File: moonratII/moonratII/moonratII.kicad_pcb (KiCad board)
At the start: 2 copper layers, 10 parts, among them Q101 IRF540N, SW101 6mm 2 Pin Tact NO, SW102 6mm 2 Pin Tact NO, SW103 6mm 2 Pin Tact NO, U101 TMP36xS

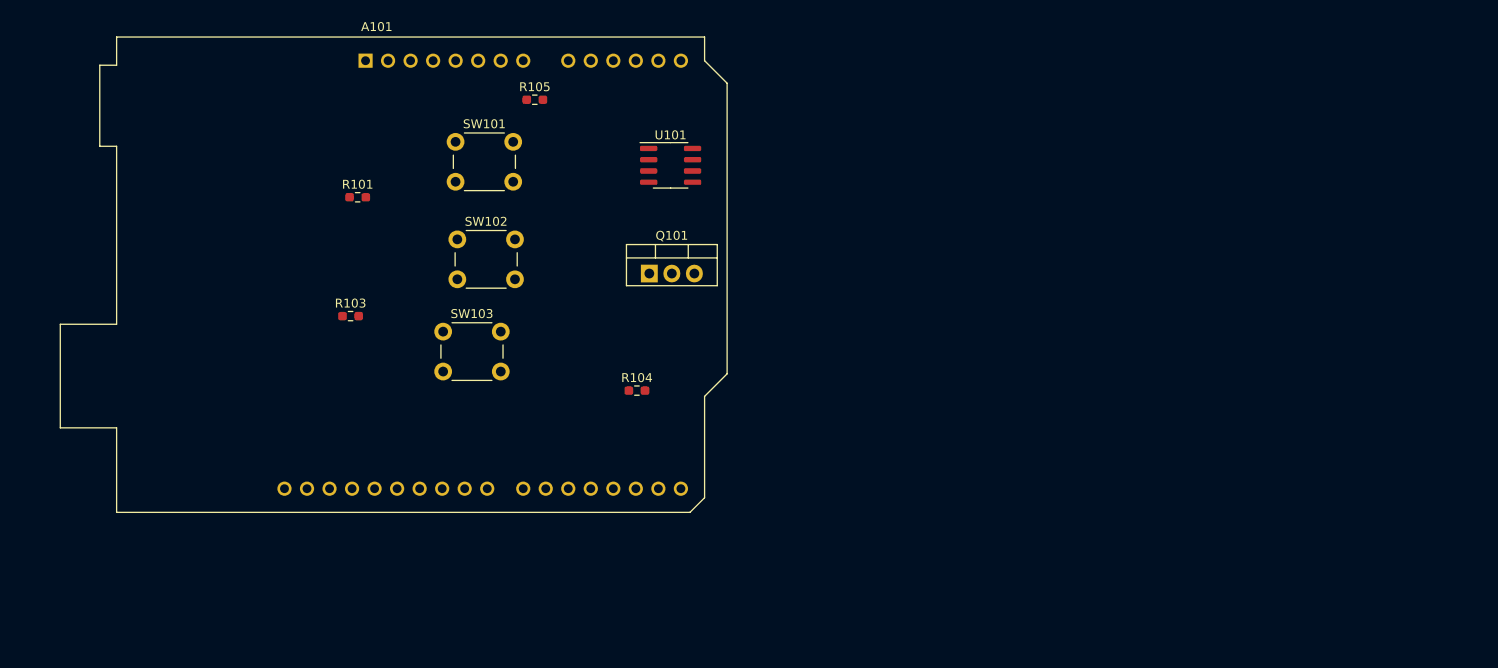
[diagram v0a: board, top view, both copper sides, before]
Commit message: Pull in parts to PCB. Make some initial placement.
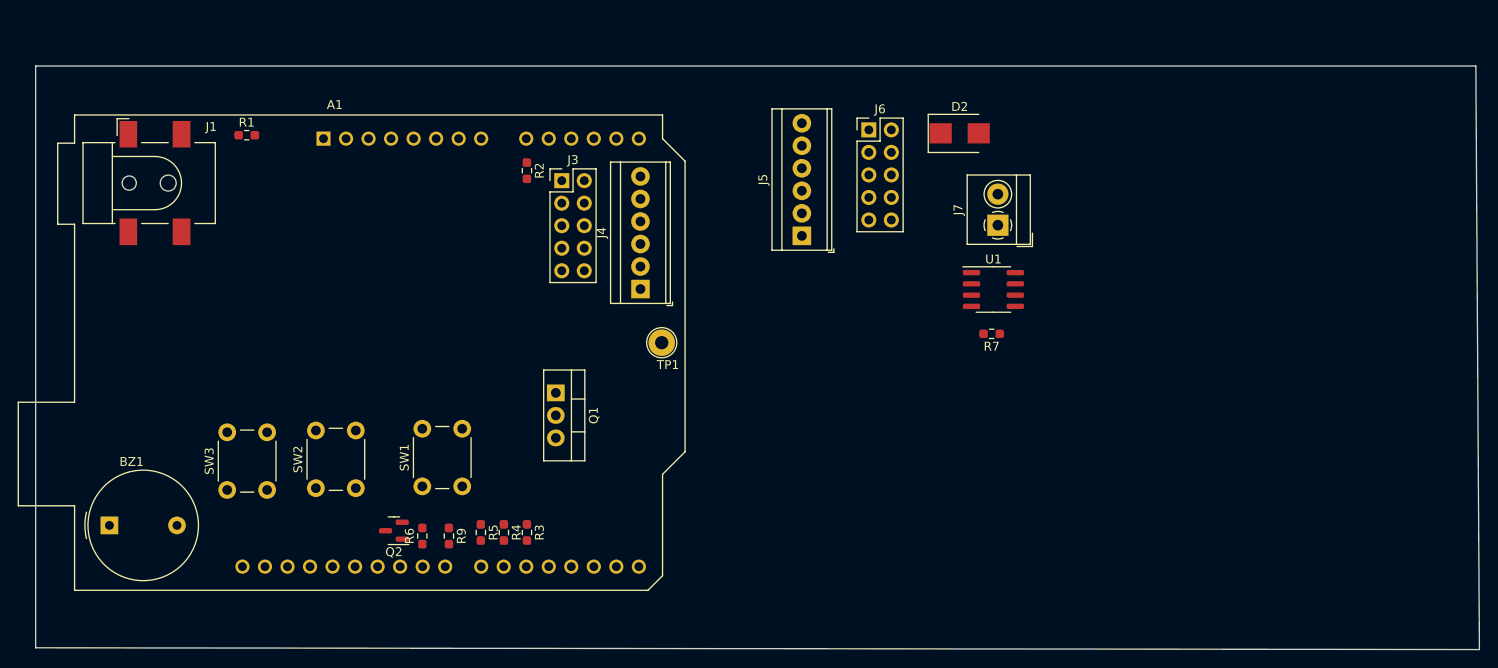
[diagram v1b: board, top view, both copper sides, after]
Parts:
- removed A101: Arduino_UNO_R3, Module:Arduino_UNO_R3
- removed Q101: IRF540N, Package_TO_SOT_THT:TO-220-3_Vertical
- removed R101: 1R, Resistor_SMD:R_0603_1608Metric_Pad0.98x0.95mm_HandSolder
- removed R103, R104, R105: 1K, Resistor_SMD:R_0603_1608Metric_Pad0.98x0.95mm_HandSolder
- removed SW101, SW102, SW103: 6mm 2 Pin Tact NO, Button_Switch_THT:SW_PUSH_6mm
- removed U101: TMP36xS, Package_SO:SOIC-8_3.9x4.9mm_P1.27mm
- added A1: Arduino_UNO_R3, Module:Arduino_UNO_R3, F.Cu at (136.3, 68.2)
- added BZ1: Buzzer_Adafruit_P1536A, GeneralPurposeAlarmDevicePCB:Buzzer_12.2mm_9.7mm_7.62mm, F.Cu at (112.1, 111.8)
- added D2: Schottky 2A, Diode_SMD:D_SMB, F.Cu at (208.0, 67.6)
- added J1: Barrel_Jack_Switch_SMT, GeneralPurposeAlarmDevicePCB:BarrelJack_CLIFF_FC681465S_SMT_Horizontal, F.Cu at (117.2, 73.2)
- added J3: Conn_02x05_Odd_Even, Connector_PinHeader_2.54mm:PinHeader_2x05_P2.54mm_Vertical, F.Cu at (163.1, 72.9)
- added J4: Screw_Terminal_01x06, TerminalBlock_TE-Connectivity:TerminalBlock_TE_282834-6_1x06_P2.54mm_Horizontal, F.Cu at (172.0, 85.2)
- added J5: Screw_Terminal_01x06, TerminalBlock_TE-Connectivity:TerminalBlock_TE_282834-6_1x06_P2.54mm_Horizontal, F.Cu at (190.2, 79.2)
- added J6: Conn_02x05_Odd_Even, Connector_PinHeader_2.54mm:PinHeader_2x05_P2.54mm_Vertical, F.Cu at (197.8, 67.2)
- added J7: Screw_Terminal_01x02, TerminalBlock_4Ucon:TerminalBlock_4Ucon_1x02_P3.50mm_Horizontal, F.Cu at (212.3, 78.0)
- added Q1: IRF520N, Package_TO_SOT_THT:TO-220-3_Vertical, F.Cu at (162.5, 96.9)
- added Q2: BSS138, Package_TO_SOT_SMD:SOT-23, F.Cu at (144.2, 112.4)
- added R1: 1R, Resistor_SMD:R_0603_1608Metric_Pad0.98x0.95mm_HandSolder, F.Cu at (127.6, 67.8)
- added R2: 1R, Resistor_SMD:R_0603_1608Metric_Pad0.98x0.95mm_HandSolder, F.Cu at (159.2, 71.8)
- added R3: 1K, Resistor_SMD:R_0603_1608Metric_Pad0.98x0.95mm_HandSolder, F.Cu at (159.2, 112.6)
- added R4: 1K, Resistor_SMD:R_0603_1608Metric_Pad0.98x0.95mm_HandSolder, F.Cu at (156.6, 112.6)
- added R5: 1K, Resistor_SMD:R_0603_1608Metric_Pad0.98x0.95mm_HandSolder, F.Cu at (154.0, 112.6)
- added R6: 1K, Resistor_SMD:R_0603_1608Metric_Pad0.98x0.95mm_HandSolder, F.Cu at (147.4, 113.0)
- added R7: 1R, Resistor_SMD:R_0603_1608Metric_Pad0.98x0.95mm_HandSolder, F.Cu at (211.6, 90.2)
- added R9: 1K, Resistor_SMD:R_0603_1608Metric_Pad0.98x0.95mm_HandSolder, F.Cu at (150.4, 113.0)
- added SW1: 6mm 2 Pin Tact NO Breadboard Friendly, Button_Switch_THT:SW_PUSH_6mm, F.Cu at (147.4, 107.4)
- added SW2: 6mm 2 Pin Tact NO Breadboard Friendly, Button_Switch_THT:SW_PUSH_6mm, F.Cu at (135.4, 107.6)
- added SW3: 6mm 2 Pin Tact NO Breadboard Friendly, Button_Switch_THT:SW_PUSH_6mm, F.Cu at (125.4, 107.8)
- added TP1: TP_GND, TestPoint:TestPoint_Loop_D2.54mm_Drill1.5mm_Beaded, F.Cu at (174.4, 91.2)
- added U1: TMP36xS, Package_SO:SOIC-8_3.9x4.9mm_P1.27mm, F.Cu at (211.8, 85.2)
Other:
- board outline added: 162.8 x 65.8 mm
